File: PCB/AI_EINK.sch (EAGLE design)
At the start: 206 parts, among them IC1 LIS3MDL, IC3 WM8960, J1 SM03B-SRSS-TBCONN_SM03B-SRSS-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, J2 C393939, J3 BM04B-SRSS-TBCONN4_BM04B-SRSS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, J4 BM04B-SRSS-TBCONN4_BM04B-SRSS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, J5 BM04B-SRSS-TBCONN4_BM04B-SRSS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, Q1 SI1308EDL-T1-GE3, Q2 DMG2307L, Q3 NMOS_C7465427, Q4 NMOS_C7465427, T1 MMUN2133LT1G, U1 TPS61092RSAR, U10 AP2112-3.3K, U11 AP2112-3.3K, U12 C233266, U13 TPD4EUSB30DQARDQA10, U14 OPA344, U15 AP2112-3.3K, U16 W25Q16JVUXIQ_TR, U17 TPD1E1B04DPYRDPY2_TEX, U18 TPD1E1B04DPYRDPY2_TEX, U19 TPD1E1B04DPYRDPY2_TEX, U2 MC74VHC1G14DFT1G, U20 TPD1E1B04DPYRDPY2_TEX, U21 TPD1E1B04DPYRDPY2_TEX, U22 TPD1E1B04DPYRDPY2_TEX, U23 TPD1E1B04DPYRDPY2_TEX, U24 TPD1E1B04DPYRDPY2_TEX, U25 DRV2605LDGSR, U3 BQ27441DRZR-G1A, U4 BQ24075, U5 MC74VHC1G14DFT1G OR C66196, U6 LSM6DS3, U7 SN74LVC244ARWPRRWP0020A, U9 EMC2301-1-ACZL-TRMSOP8_MC_MCH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, Y1 ABM8-272-T3

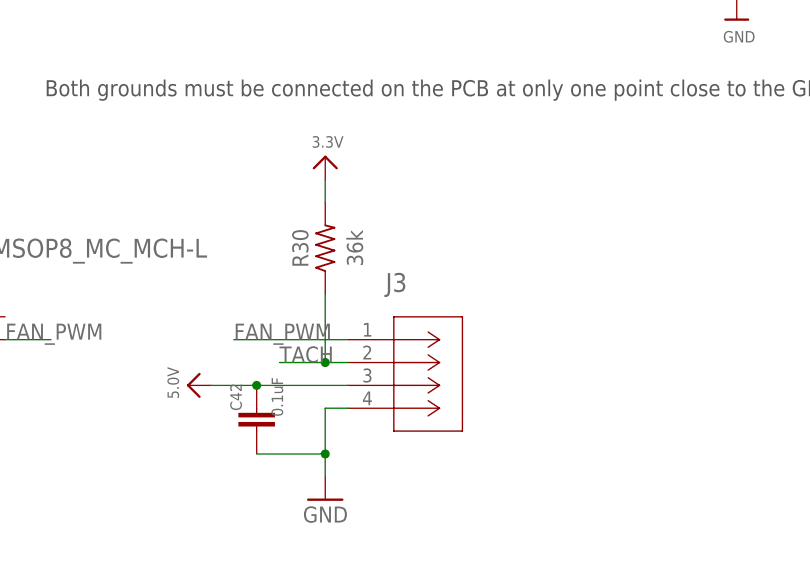
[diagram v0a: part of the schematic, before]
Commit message: v0.7
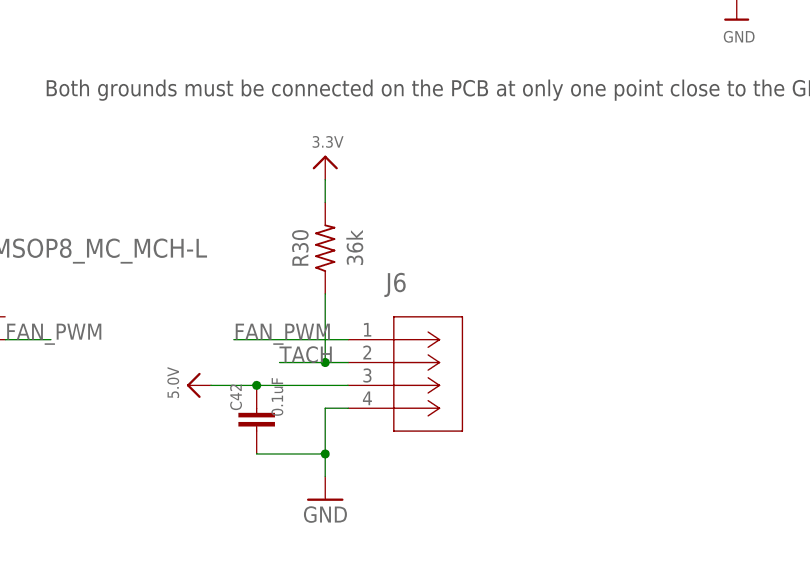
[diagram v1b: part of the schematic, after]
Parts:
- removed J3: BM04B-SRSS-TBCONN4_BM04B-SRSS_JST, 2024-05-18_10-24-10_Library:BM04B-SRSS-TBCONN4_BM04B-SRSS_JST
- added J6: SM04B-SRSS-TBCONN_SM04B-SRSS-TB_JST, 2024-06-16_01-36-12_Library:SM04B-SRSS-TBCONN_SM04B-SRSS-TB_JST
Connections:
- net 5.0V: now also J6.3; no longer J3.3
- net FAN_PWM: now also J6.1; no longer J3.1
- net GND: now also J6.4; no longer J3.4
- net TACH: now also J6.2; no longer J3.2
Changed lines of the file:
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@@
 <part name="L3" library="LQH5BPN2R2NT0L" deviceset="LQH5BPN2R2NT0L" device="" value="FNR5012S100MT 10uH"/>
 <part name="U7" library="2024-05-18_09-46-26_Library" deviceset="SN74LVC244ARWPR" device="RWP0020A"/>
-<part name="J3" library="2024-05-18_10-24-10_Library" deviceset="BM04B-SRSS-TB" device="CONN4_BM04B-SRSS_JST"/>
 <part name="J4" library="2024-05-18_10-24-10_Library" deviceset="BM04B-SRSS-TB" device="CONN4_BM04B-SRSS_JST"/>
 <part name="J5" library="2024-05-18_10-24-10_Library" deviceset="BM04B-SRSS-TB" device="CONN4_BM04B-SRSS_JST"/>
@@
 <part name="U$111" library="microbuilder" deviceset="GND" device=""/>
 <part name="U$112" library="microbuilder" deviceset="GND" device=""/>
+<part name="J6" library="2024-06-16_01-36-12_Library" deviceset="SM04B-SRSS-TB" device="CONN_SM04B-SRSS-TB_JST"/>
 </parts>
 <sheets>
@@
 <attribute name="VALUE" x="632.1752" y="-36.6014" size="2.083" layer="96" ratio="6"/>
 </instance>
-<instance part="J3" gate="A" x="548.64" y="152.4" smashed="yes">
-<attribute name="NAME" x="552.8046" y="157.7086" size="2.083" layer="95" ratio="6"/>
-</instance>
 <instance part="J4" gate="A" x="937.26" y="241.3" smashed="yes">
 <attribute name="NAME" x="941.4246" y="246.6086" size="2.083" layer="95" ratio="6"/>
@@
 <attribute name="VALUE" x="-42.164" y="182.88" size="1.27" layer="96"/>
 </instance>
+<instance part="J6" gate="A" x="548.64" y="152.4" smashed="yes">
+<attribute name="NAME" x="552.8046" y="157.7086" size="2.083" layer="95" ratio="6"/>
+</instance>
 </instances>
 <busses>
@@
 <pinref part="C42" gate="G$1" pin="2"/>
 <wire x1="546.1" y1="139.7" x2="538.48" y2="139.7" width="0.1524" layer="91"/>
-<pinref part="J3" gate="A" pin="4"/>
+<pinref part="J6" gate="A" pin="4"/>
 </segment>
 <segment>
@@
 <wire x1="538.48" y1="147.32" x2="533.4" y2="147.32" width="0.1524" layer="91"/>
 <junction x="538.48" y="147.32"/>
-<pinref part="J3" gate="A" pin="3"/>
+<pinref part="J6" gate="A" pin="3"/>
 </segment>
 <segment>
@@
 <wire x1="546.1" y1="149.86" x2="546.1" y2="157.48" width="0.1524" layer="91"/>
 <junction x="546.1" y="149.86"/>
-<pinref part="J3" gate="A" pin="2"/>
+<pinref part="J6" gate="A" pin="2"/>
 </segment>
 </net>
@@
 <wire x1="548.64" y1="152.4" x2="535.94" y2="152.4" width="0.1524" layer="91"/>
 <label x="535.94" y="152.4" size="1.778" layer="95"/>
-<pinref part="J3" gate="A" pin="1"/>
+<pinref part="J6" gate="A" pin="1"/>
 </segment>
 </net>

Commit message: before modification, v0.7, for fateen and adam
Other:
- note added: "ACTIVE COOLING"
- note added: "AUDIO SUBSYSTEM"
- note added: "CAMERA"
- note added: "DIGITAL PERIPHERAL"
- note added: "EINK_SUBSYSTEM"
- note added: "HAPTIC MOTOR"
- note added: "MOTION SUBSYSTEM"
- note added: "PCIE M.2"
- note added: "POWER SUBSYSTEM"
- note added: "SAM"
- note added: "SOM"
- note added: "USB2.0"
- note removed: "CAMERA MODULE"
- note removed: "EINK HiGH VOLTAGE MODULE"
- moved on the sheet: BUD, BUP, BUS, C1, C10, C11, C12, C13, C14, C15, C16, C17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
